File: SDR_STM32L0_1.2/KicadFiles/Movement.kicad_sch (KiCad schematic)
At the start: 5 parts, among them U6 BMI323

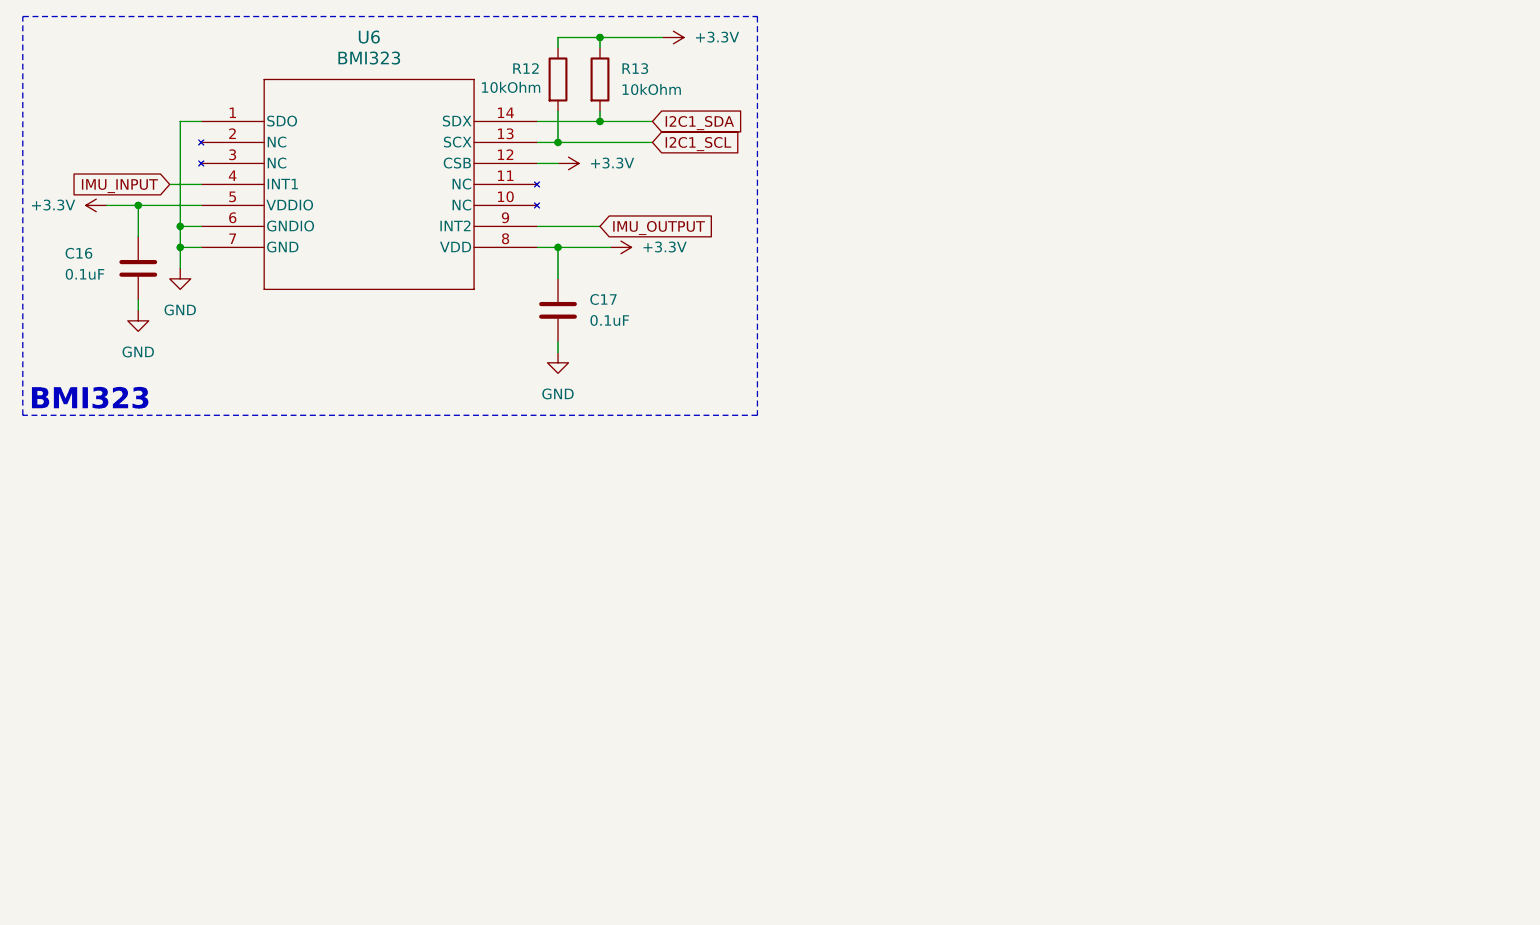
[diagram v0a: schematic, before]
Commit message: dev
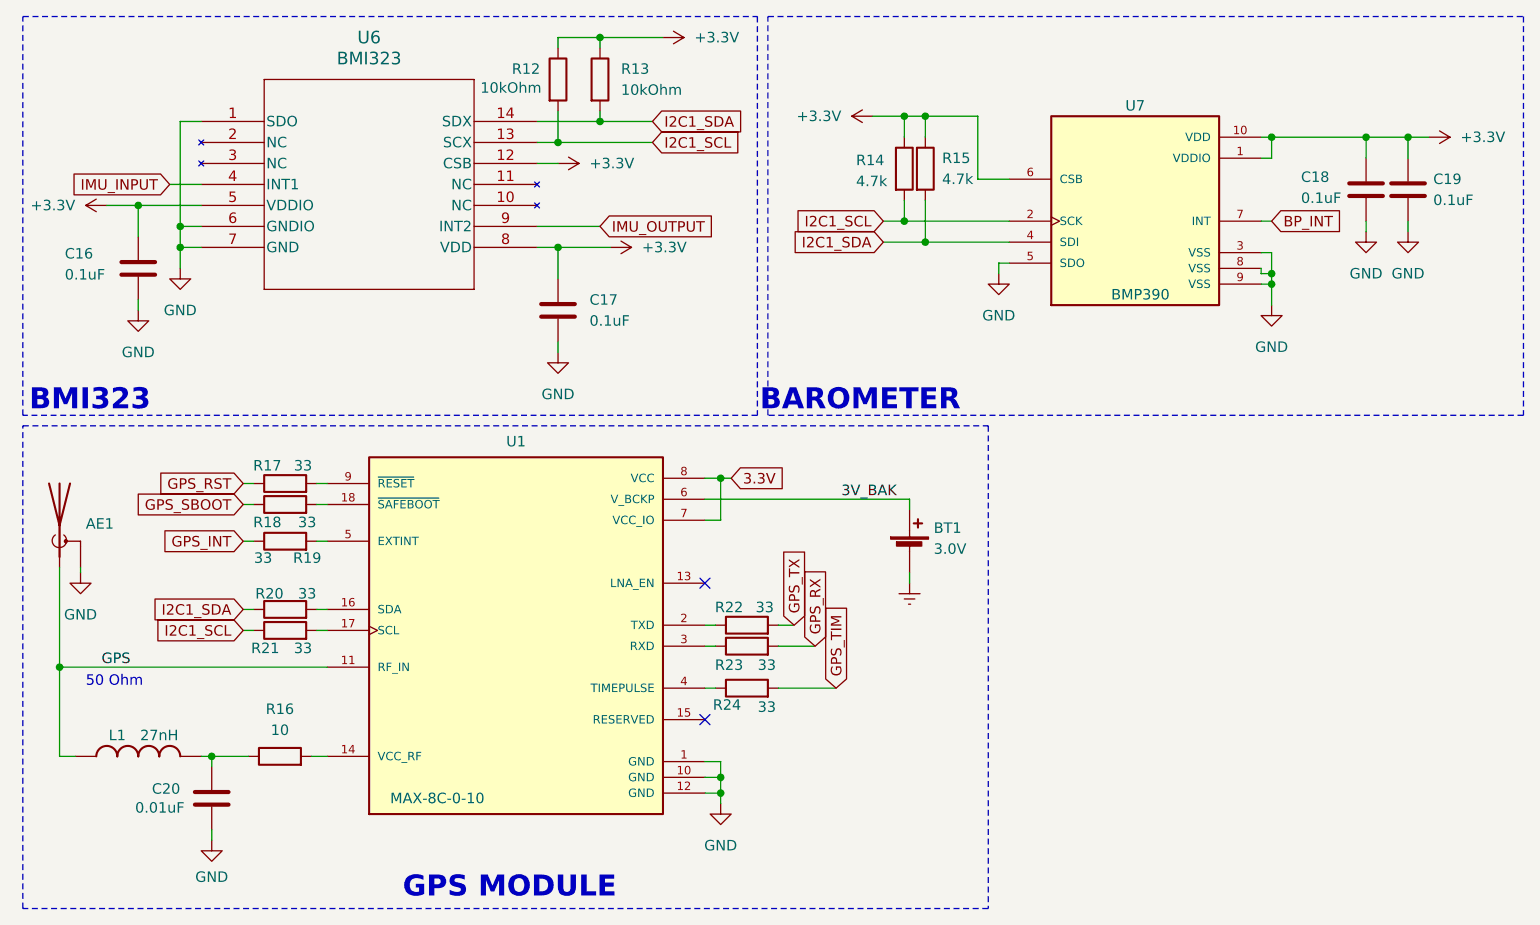
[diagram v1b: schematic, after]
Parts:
- added AE1: 0734120110, Flight-Computer:73412-0110, symbol Flight-Computer:0734120110
- added BT1: MS614SE-FL28E, Flight-Computer:MS621FE-FL11E, symbol Flight-Computer:MS614SE-FL28E
- added C18, C19: 0.1uF, symbol Device:C
- added C20: 0.01uF, symbol Device:C
- added L1: 27nH, Flight-Computer:L-07C27NJV6T, symbol Flight-Computer:L-07C27NJV6T
- added R14, R15: 4.7k, symbol Device:R
- added R16: 10, symbol Device:R
- added R17, R18, R19, R20, R21, R22, R23, R24: 33, symbol Device:R
- added U1: MAX-8C-0-10, Flight-Computer:MAX-8C-0, symbol Flight-Computer:MAX-8C-0-10
- added U7: BMP390, Flight-Computer:BMP390, symbol Flight-Computer:BMP390
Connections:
- net +3.3V: now also C18.1, C19.1, R14.1, R15.1, U7.1 (VDDIO), U7.10 (VDD), U7.6 (CSB)
- net GND: now also AE1.2 (Shield), C18.2, C19.2, C20.2, U1.1 (GND), U1.10 (GND), U1.12 (GND), U7.3 (VSS), U7.5 (SDO), U7.8 (VSS), U7.9 (VSS)
- net I2C1_SCL: now also R14.2, R21.1, U7.2 (SCK)
- net I2C1_SDA: now also R15.2, R20.1, U7.4 (SDI)
- new net: C20.1, L1.2, R16.1
- new net: R16.2, U1.14 (VCC_RF)
- new net: R24.1, U1.4 (TIMEPULSE)
- new net: R23.1, U1.3 (RXD)
- new net: R17.2, U1.9 (~{RESET})
- new net: R21.2, U1.17 (SCL)
- new net: R18.2, U1.18 (~{SAFEBOOT})
- new net: R19.2, U1.5 (EXTINT)
- new net: R20.2, U1.16 (SDA)
- new net: R22.1, U1.2 (TXD)
- new net 3.3V: U1.7 (VCC_IO), U1.8 (VCC)
- new net 3V_BAK: BT1.1 (+), U1.6 (V_BCKP)
- new net BP_INT: U7.7 (INT)
- new net Earth: BT1.2 (-)
- new net GPS: AE1.1 (A), L1.1, U1.11 (RF_IN)
- new net GPS_INT: R19.1
- new net GPS_RST: R17.1
- new net GPS_RX: R23.2
- new net GPS_SBOOT: R18.1
- new net GPS_TIM: R24.2
- new net GPS_TX: R22.2
- no-connect marks 0 -> 2
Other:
- note added: "50 Ohm"
- note added: "BAROMETER"
- note added: "GPS MODULE"

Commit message: dev
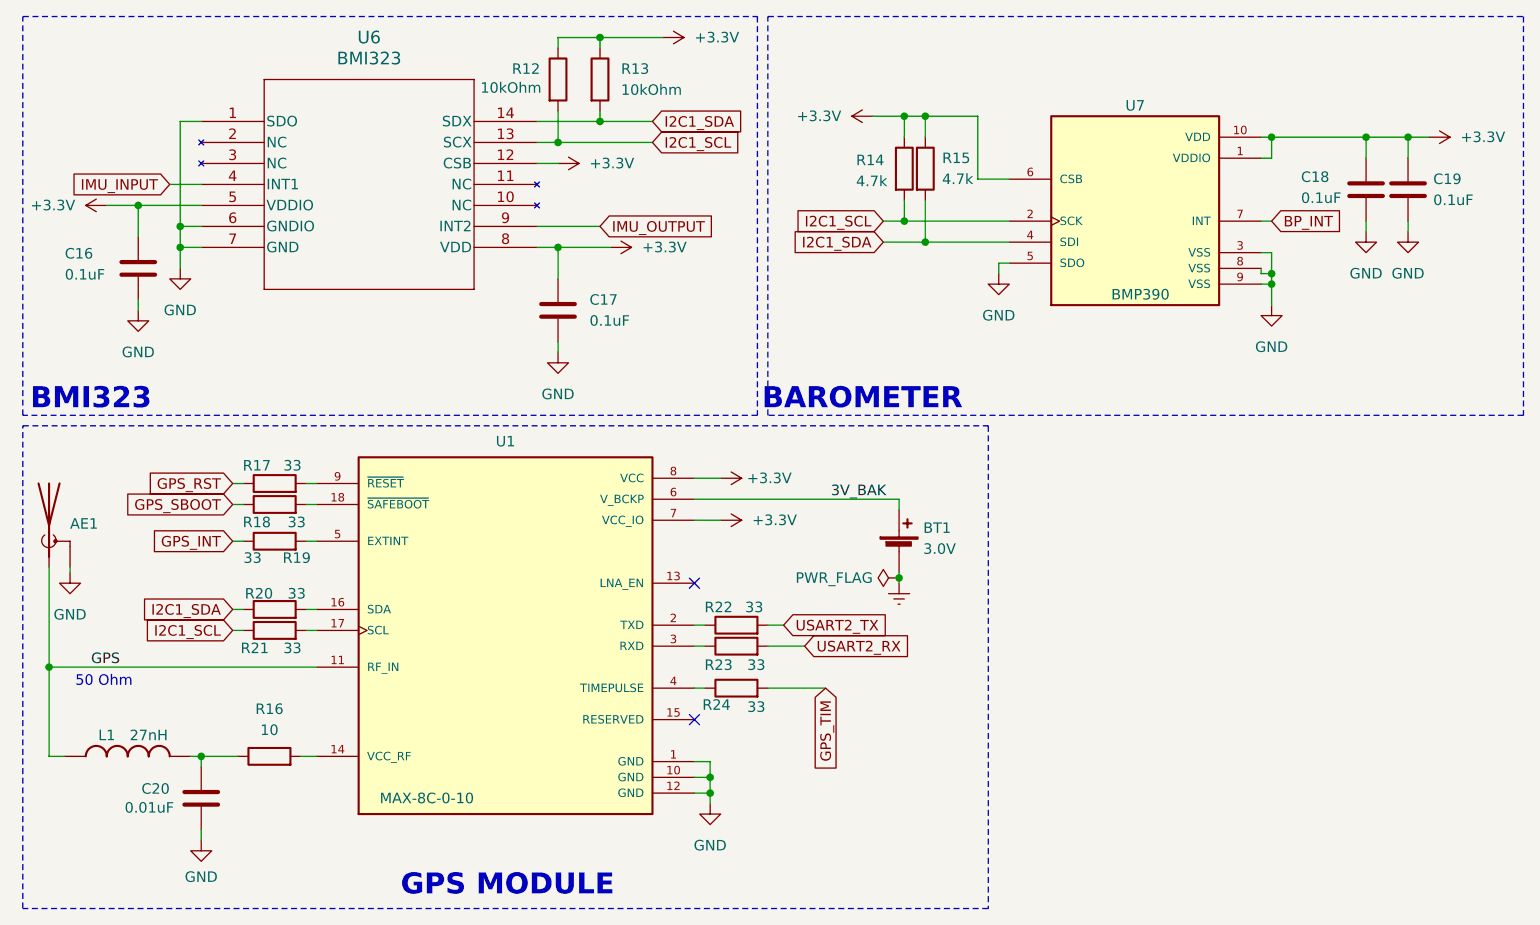
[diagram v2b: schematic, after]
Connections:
- net 3.3V is gone; now on net +3.3V: U1.7 (VCC_IO), U1.8 (VCC)
- net GPS_RX renamed USART2_RX
- net GPS_TX renamed USART2_TX
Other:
- moved on the sheet: AE1, BT1, C20, L1, R16, R17, R18, R19, R20, R21, R22, R23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

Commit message: added 1.2 back
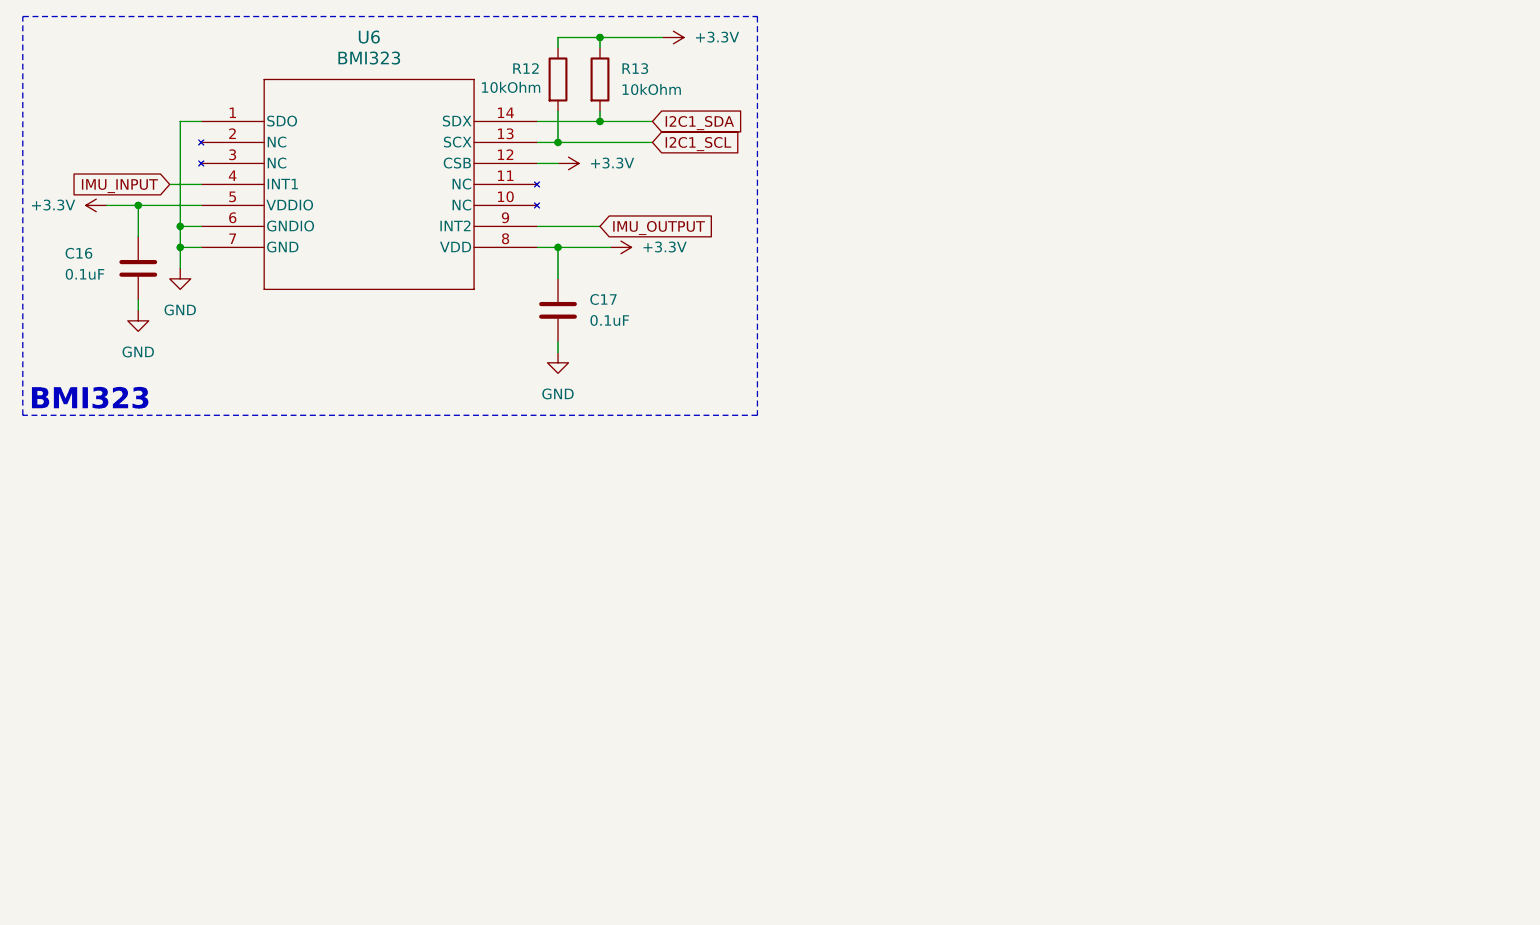
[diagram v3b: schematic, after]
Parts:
- removed AE1: 0734120110, Flight-Computer:73412-0110, symbol Flight-Computer:0734120110
- removed BT1: MS614SE-FL28E, Flight-Computer:MS621FE-FL11E, symbol Flight-Computer:MS614SE-FL28E
- removed C18, C19: 0.1uF, symbol Device:C
- removed C20: 0.01uF, symbol Device:C
- removed L1: 27nH, Flight-Computer:L-07C27NJV6T, symbol Flight-Computer:L-07C27NJV6T
- removed R14, R15: 4.7k, symbol Device:R
- removed R16: 10, symbol Device:R
- removed R17, R18, R19, R20, R21, R22, R23, R24: 33, symbol Device:R
- removed U1: MAX-8C-0-10, Flight-Computer:MAX-8C-0, symbol Flight-Computer:MAX-8C-0-10
- removed U7: BMP390, Flight-Computer:BMP390, symbol Flight-Computer:BMP390
- U6: footprint USBs:BMI323 -> Connector_USB:BMI323
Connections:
- no-connect marks 2 -> 0
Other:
- note removed: "50 Ohm"
- note removed: "BAROMETER"
- note removed: "GPS MODULE"
